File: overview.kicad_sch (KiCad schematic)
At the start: 0 parts

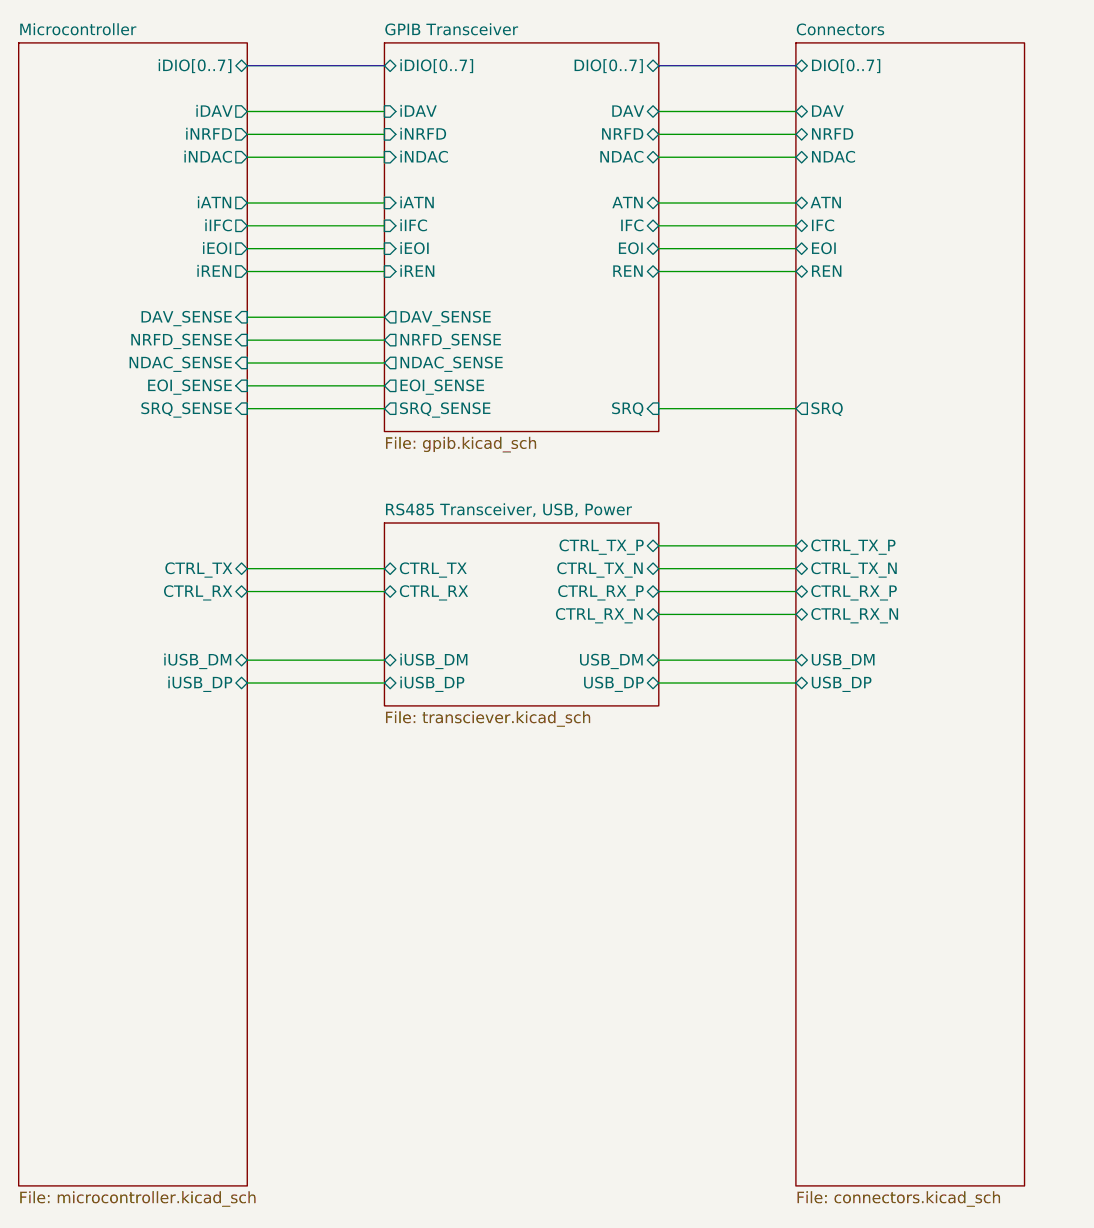
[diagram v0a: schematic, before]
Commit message: Finish up schematics
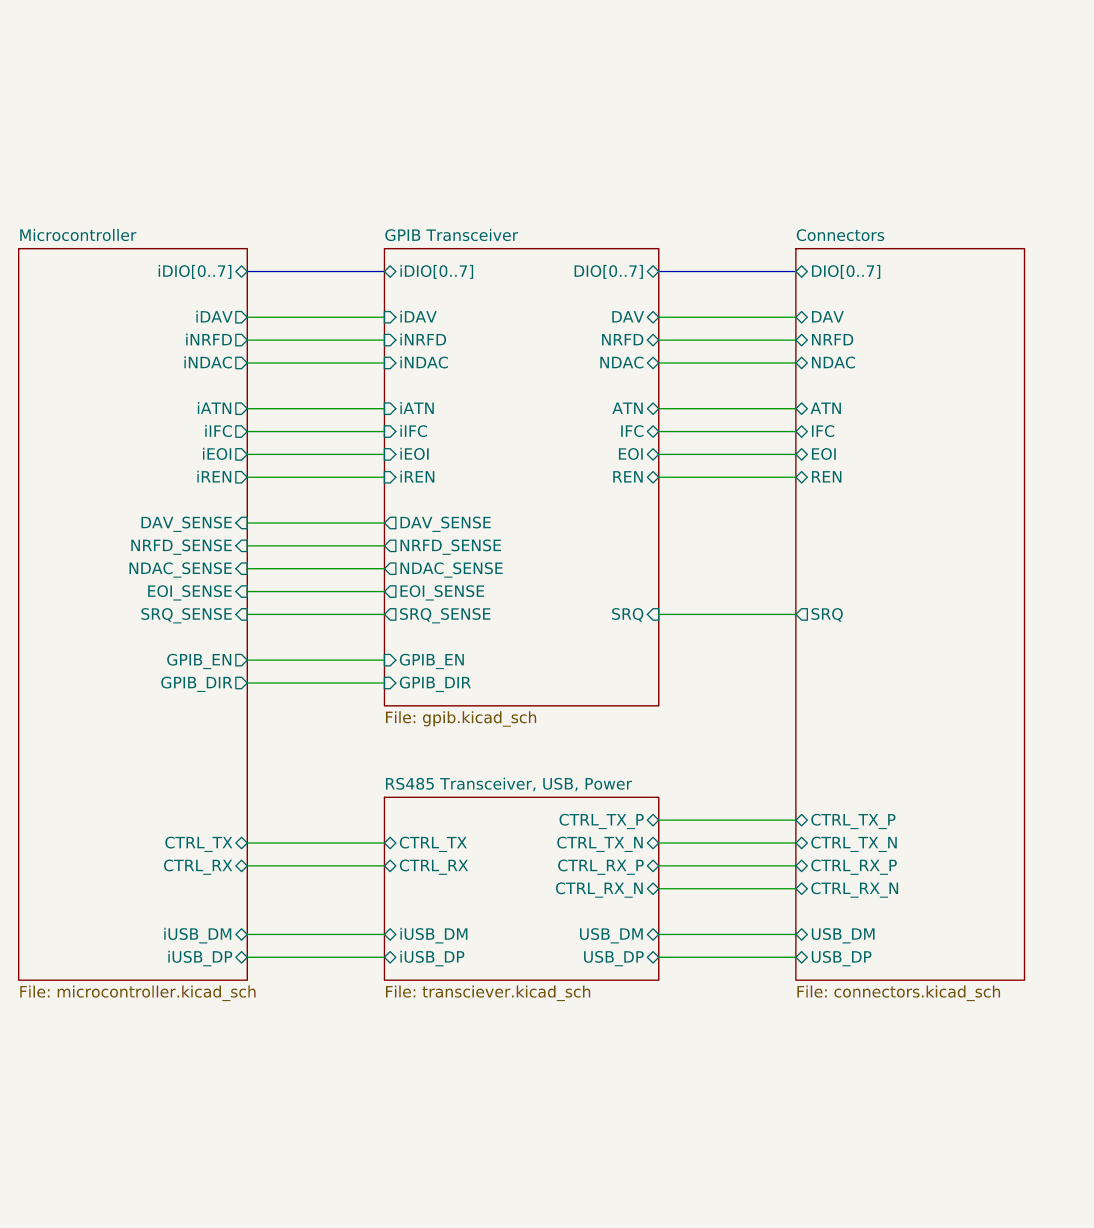
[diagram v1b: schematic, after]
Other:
- sheet GPIB Transceiver ports: added GPIB_DIR, GPIB_EN; removed none
- sheet Microcontroller ports: added GPIB_DIR, GPIB_EN; removed none
